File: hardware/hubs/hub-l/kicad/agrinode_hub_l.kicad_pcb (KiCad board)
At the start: 2 copper layers, 130 x 96 mm, 105 parts, among them J1 DC 12V 5.5/2.1, J2 DC IN 7-24V, J3 SOLAR 6-24V, J4 USB 5V / PROG, J5 BAT NTC 10k, J6 PROG, J7 I2C, J8 LED STRIP WS2813, J9 RS-485, Q1 AO3401A, Q2 AO3401A, Q3 MMBT3904, Q4 MMBT3904, Q5 BSS138, Q6 MMBT3904, SW1 RESET, SW2 BOOT / PAIR, U1 LM2596S-5.0, U2 TP4056, U3 MIC29302WU, U4 ESP32-WROOM-32E-N8, U5 CH340C, U6 DS3231MZ, U7 MAX3485ESA, U8 Ra-02 SX1278 433MHz

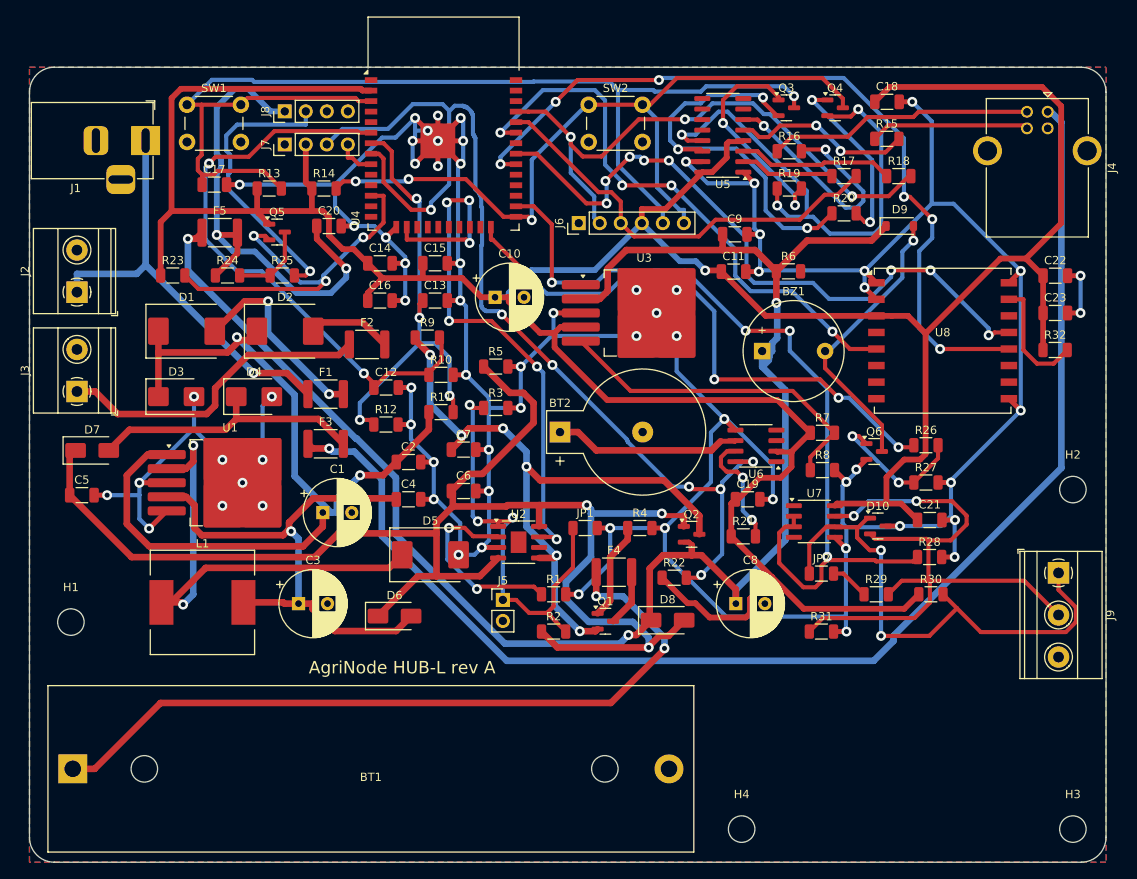
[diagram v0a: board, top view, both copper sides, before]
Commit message: hubs: routing progress snapshot
Co-Authored-By: Claude Opus 5.5 <noreply@anthropic.com>
Claude-Session: https://claude.ai/code/session_014J7amXZ5Y6AZWEh5CjDNja
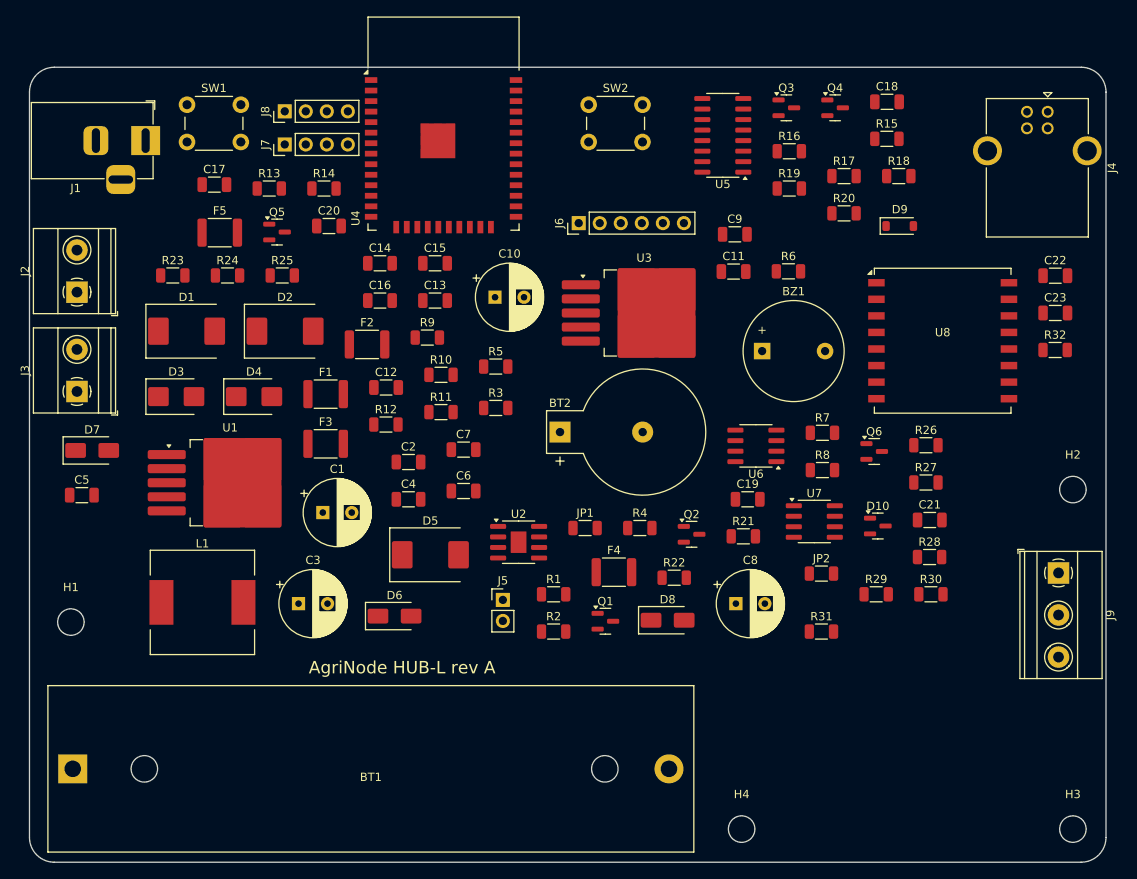
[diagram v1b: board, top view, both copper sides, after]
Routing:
- net GND: track 554.7 -> 0.00 mm, vias 68 -> 0
- net +3V3: track 411.2 -> 0.00 mm, vias 1 -> 0
- net VSYS: track 201.4 -> 0.00 mm, vias 3 -> 0
- net /Power - 12V, solar and USB inputs, 18650 charger, rails/V5: track 183.3 -> 0.00 mm, vias 3 -> 0
- net /Power - 12V, solar and USB inputs, 18650 charger, rails/VUSB_RAW: track 159.8 -> 0.00 mm, vias 1 -> 0
- net /ESP32, programming, buttons, RTC, LED strip, buzzer/ESP_EN: track 139.1 -> 0.00 mm, vias 1 -> 0
- net /ESP32, programming, buttons, RTC, LED strip, buzzer/I2C_SCL: track 128.1 -> 0.00 mm, vias 7 -> 0
- net /Power - 12V, solar and USB inputs, 18650 charger, rails/VIN_BUCK: track 106.5 -> 0.00 mm, vias 2 -> 0
- net RS485_DE: track 101.8 -> 0.00 mm, vias 4 -> 0
- net SPI_SCK: track 95.7 -> 0.00 mm, vias 6 -> 0
- net /ESP32, programming, buttons, RTC, LED strip, buzzer/BOOT_BTN: track 93.9 -> 0.00 mm, vias 3 -> 0
- net /Power - 12V, solar and USB inputs, 18650 charger, rails/BATT_CELL: track 92.1 -> 0.00 mm, vias 2 -> 0
- net SPI_MISO: track 81.6 -> 0.00 mm, vias 8 -> 0
- net /Power - 12V, solar and USB inputs, 18650 charger, rails/VBAT: track 80.4 -> 0.00 mm, vias 6 -> 0
- net /RS-485 and uplink/RS485_B: track 77.7 -> 0.00 mm, vias 2 -> 0
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- removed copper zone on B.Cu, net GND
- removed copper zone on F.Cu, net GND
